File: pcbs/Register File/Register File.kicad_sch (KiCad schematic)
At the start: 1 part

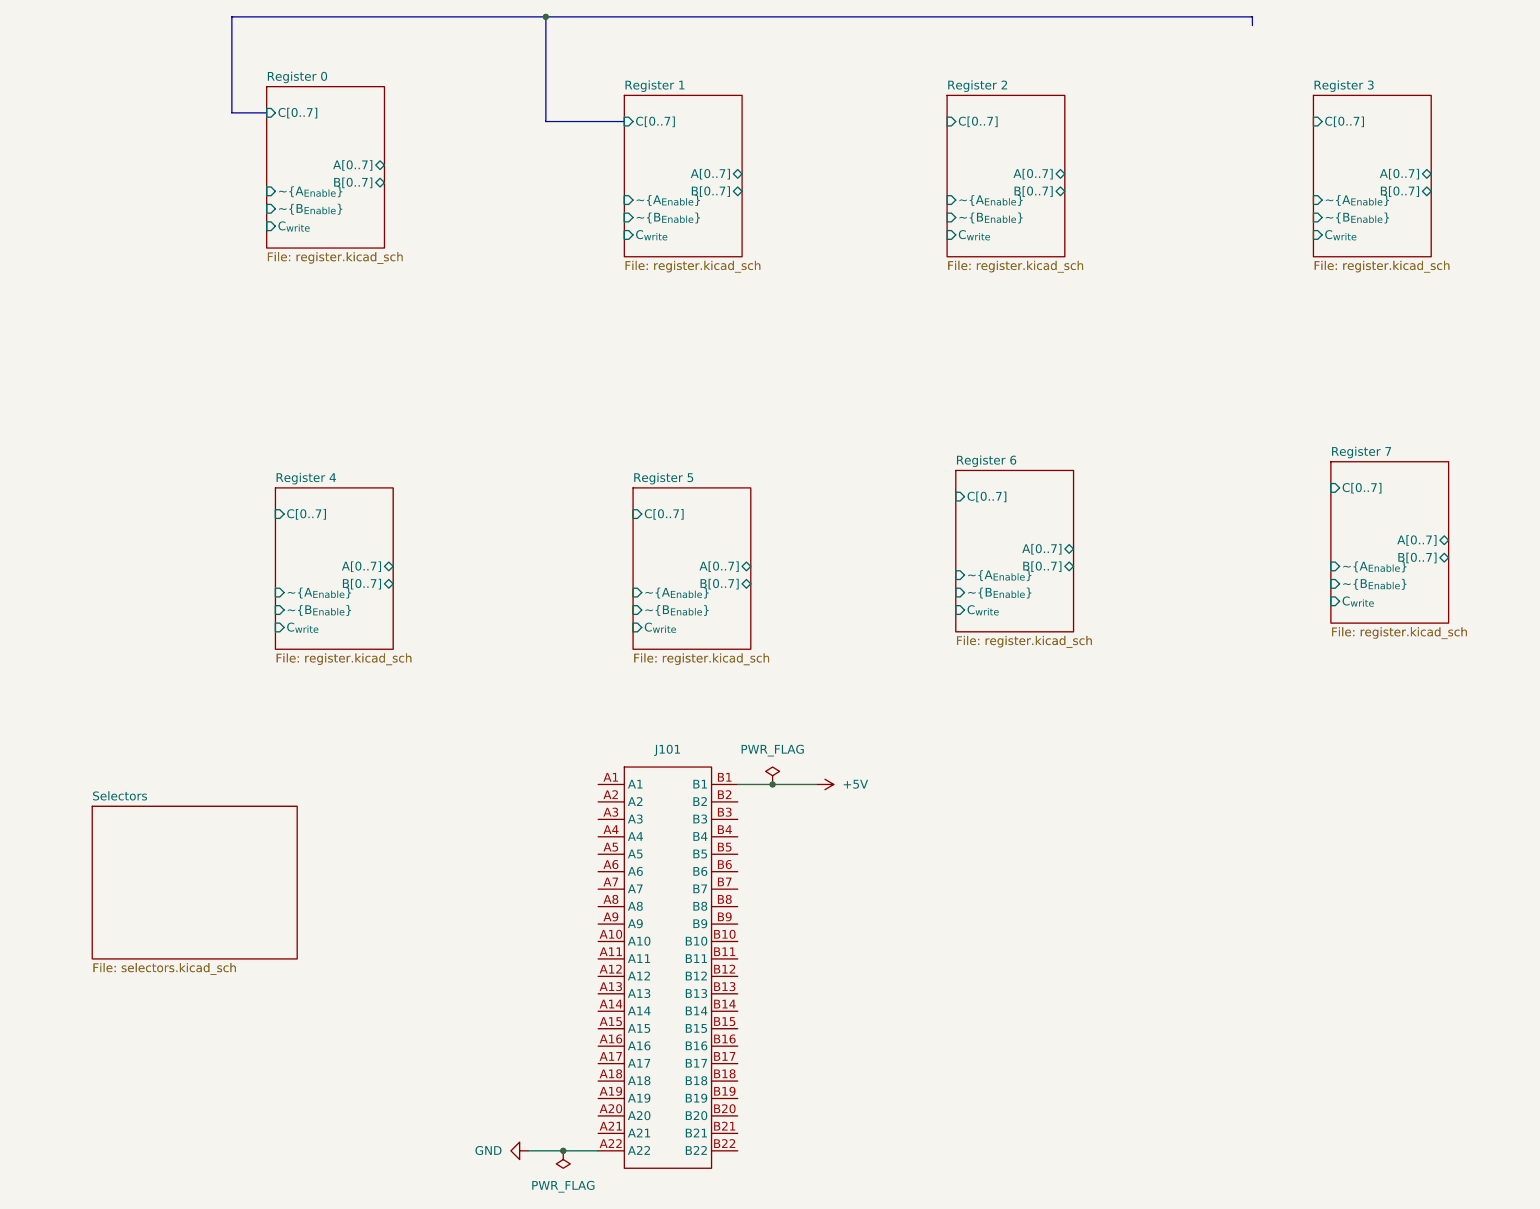
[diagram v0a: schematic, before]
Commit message: Roughing out some layout
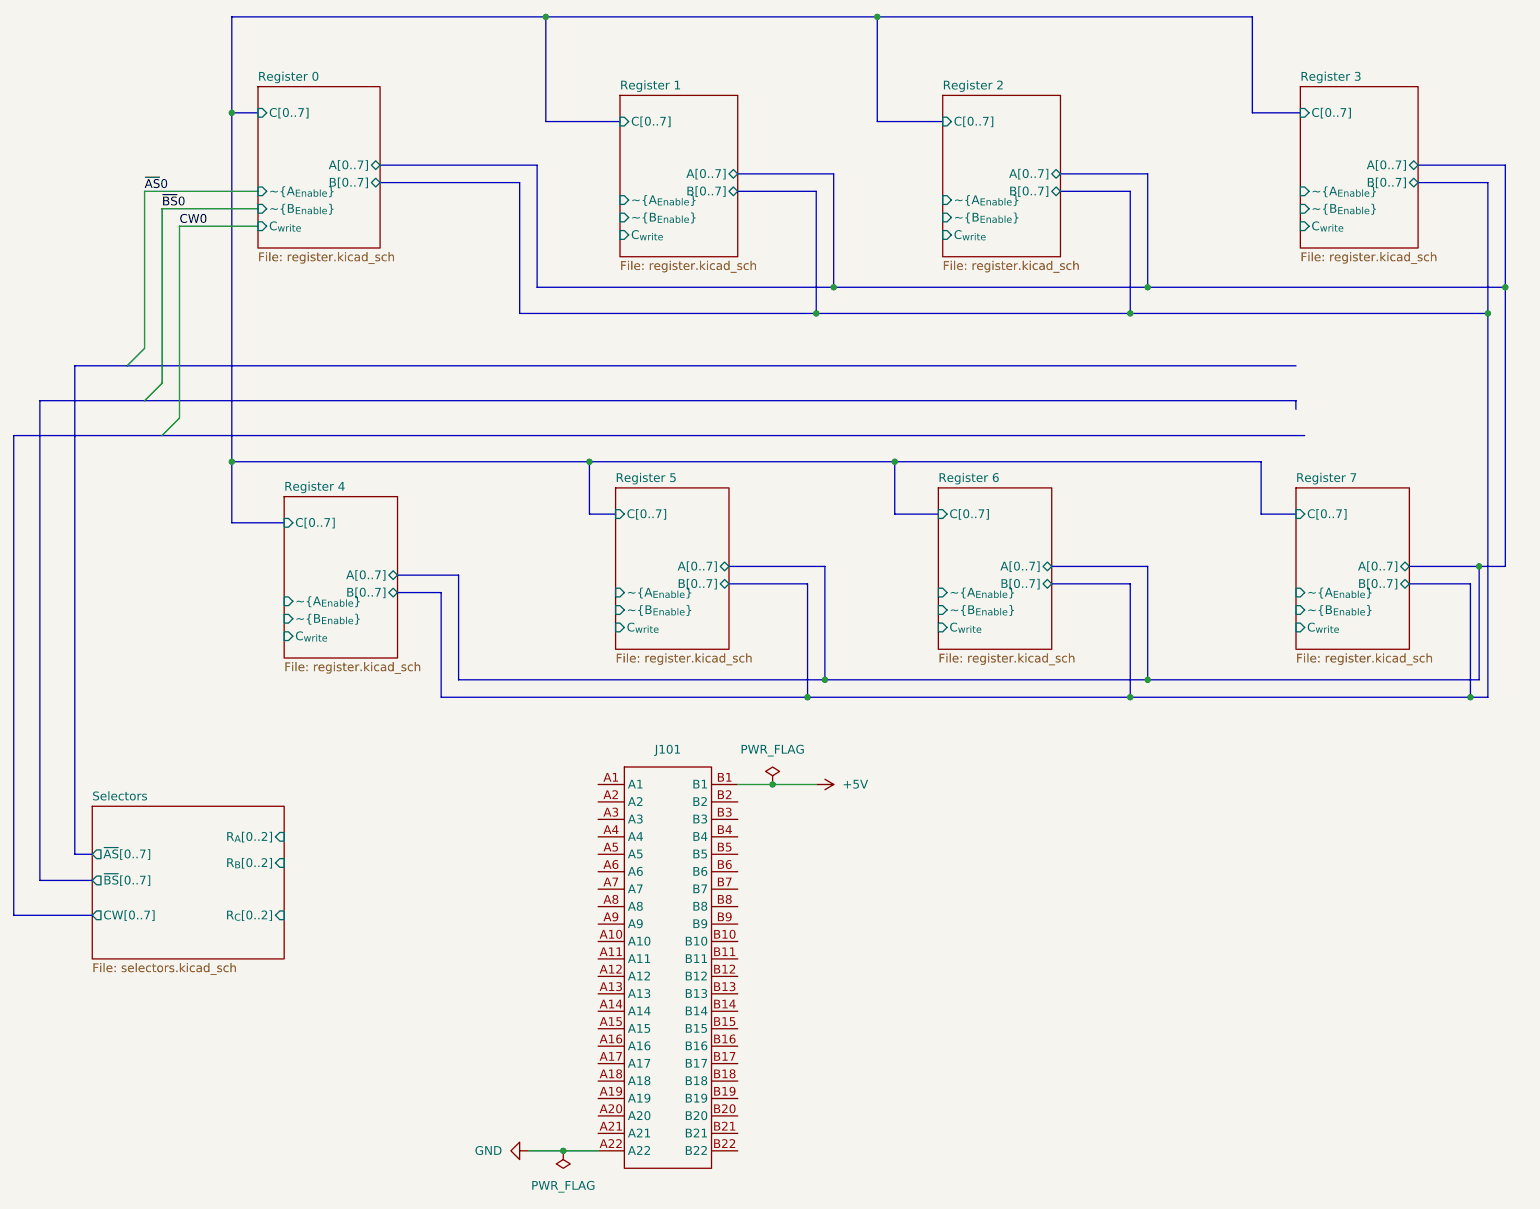
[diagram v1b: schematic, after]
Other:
- sheet Selectors ports: added CW[0..7], R_{A}[0..2], R_{B}[0..2], R_{C}[0..2], ~{AS}[0..7], ~{BS}[0..7]; removed none
